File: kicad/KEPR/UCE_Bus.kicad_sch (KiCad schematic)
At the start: 1 part, among them J11 10141995-005RLF

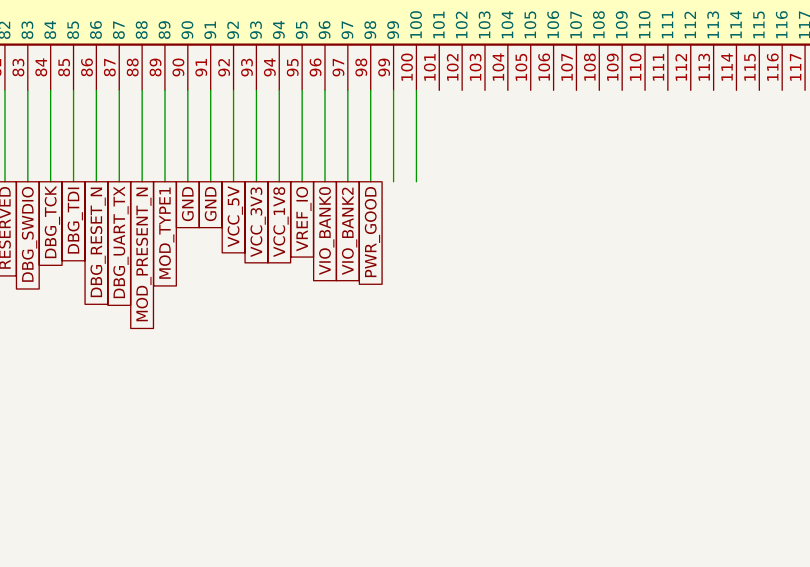
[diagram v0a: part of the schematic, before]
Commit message: Ajustes no Power Rail, entre outros ajustes.
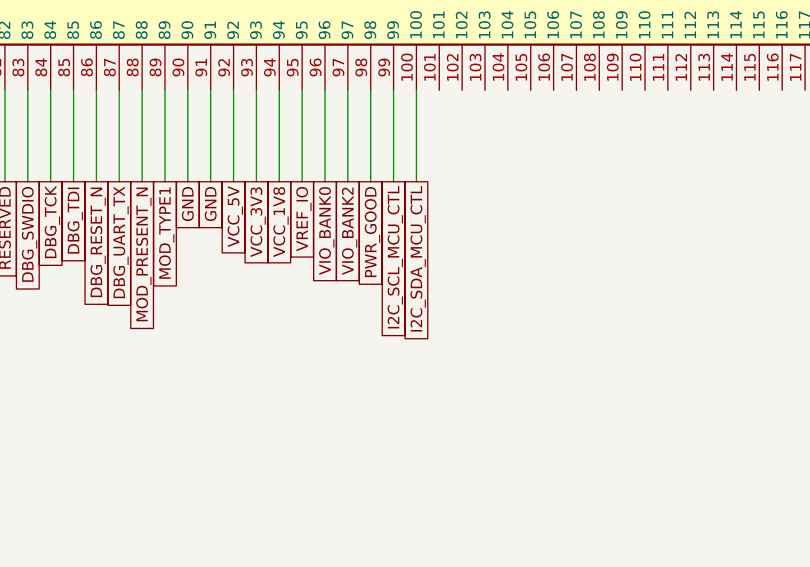
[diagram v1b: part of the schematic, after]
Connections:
- net I2C_SDA_MCU_CTL: now reaches J11.100
- net I2C_SCL_MCU_CTL: now reaches J11.99
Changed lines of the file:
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@@
+		)
+	)
+	(global_label "I2C_SDA_MCU_CTL"
+		(shape passive)
+		(at 297.18 83.82 270)
+		(fields_autoplaced yes)
+		(effects
+			(font
+				(size 1.27 1.27)
+			)
+			(justify right)
+		)
+		(property "Intersheetrefs" "${INTERSHEET_REFS}"
+			(at 297.18 102.5667 90)
+			(effects
+				(font
+					(size 1.27 1.27)
+				)
+				(justify right)
+				(hide yes)
+			)
 		)
 	)
@@
 				(hide yes)
 			)
+		)
+	)
+	(global_label "I2C_SCL_MCU_CTL"
+		(shape passive)
+		(at 294.64 83.82 270)
+		(fields_autoplaced yes)
+		(effects
+			(font
+				(size 1.27 1.27)
+			)
+			(justify right)
+		)
+		(property "Intersheetrefs" "${INTERSHEET_REFS}"
+			(at 294.64 102.5062 90)
+			(effects
+				(font
+					(size 1.27 1.27)
+				)
+				(justify right)
+				(hide yes)
+			)
